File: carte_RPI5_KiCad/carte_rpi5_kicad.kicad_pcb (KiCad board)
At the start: 2 copper layers, 25 parts, among them J0 Vin batterie, J1 Conn_01x03, J2 Conn_01x03, J3 Conn_01x03, J4 Conn_01x03, J5 Conn_01x03, J6 Conn_01x03, J7 Conn_01x03, J8 Conn_01x03, SW1 SW_SPDT

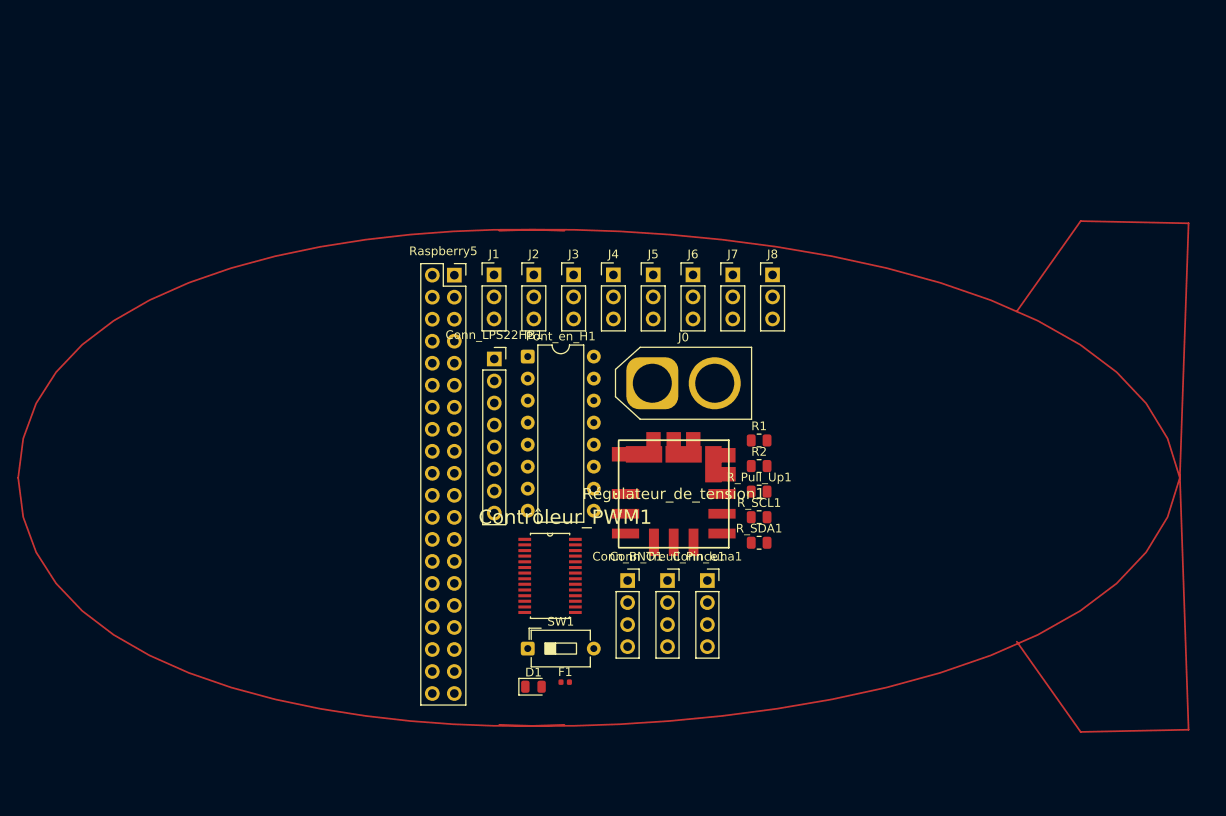
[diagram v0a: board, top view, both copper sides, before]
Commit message: mise à jour PCB
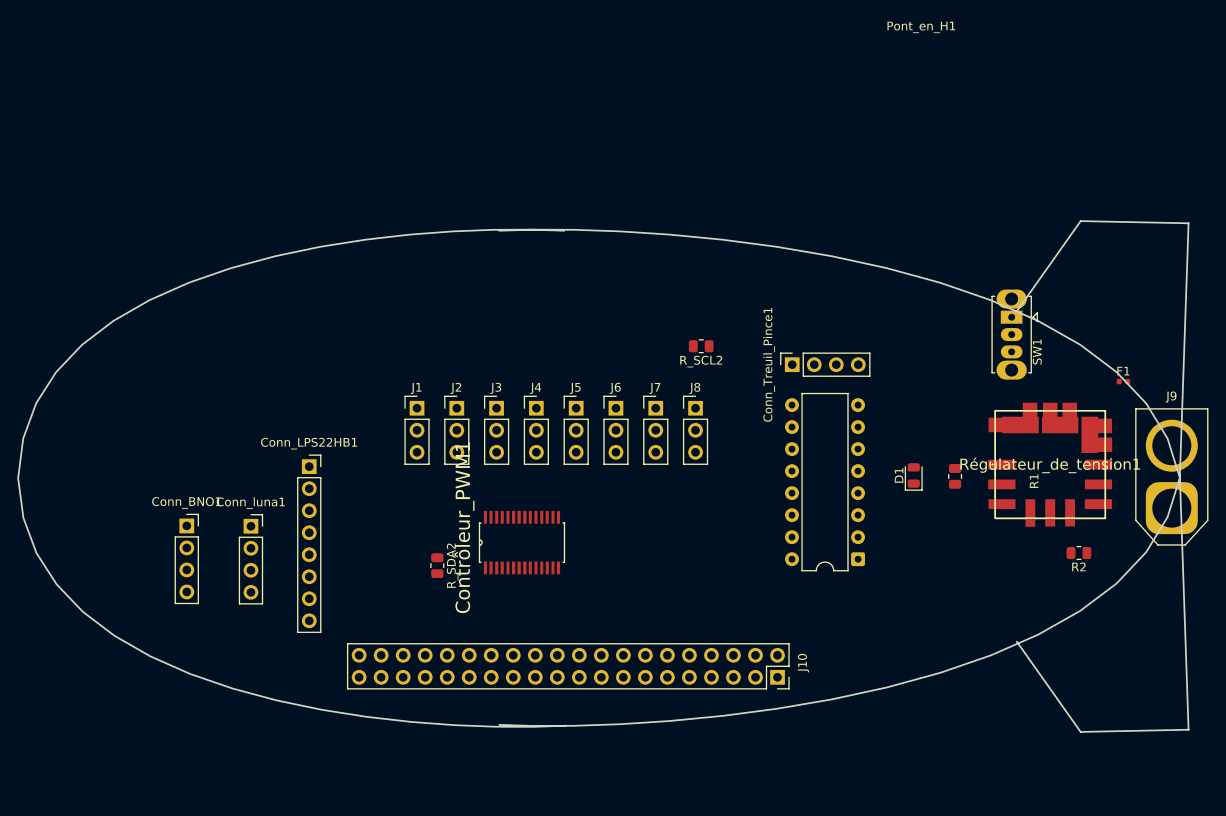
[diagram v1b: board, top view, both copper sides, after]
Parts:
- removed J0: Vin batterie, Connector_AMASS:AMASS_XT60-F_1x02_P7.20mm_Vertical
- removed R_Pull_Up1: 1 k, Resistor_SMD:R_0805_2012Metric
- removed R_SCL1, R_SDA1: 4,7k, Resistor_SMD:R_0805_2012Metric
- removed Raspberry5: CM5108032, Connector_PinSocket_2.54mm:PinSocket_2x20_P2.54mm_Vertical
- added J10: RPI5_40pins, Connector_PinSocket_2.54mm:PinSocket_2x20_P2.54mm_Vertical, F.Cu at (143.6, 109.0)
- added J9: XT60-M, Connector_AMASS:AMASS_XT60-F_1x02_P7.20mm_Vertical, F.Cu at (189.1, 89.5)
- added R_SCL2: 4,7k, Resistor_SMD:R_0805_2012Metric, F.Cu at (134.8, 70.8)
- added R_SDA2: 4,7k, Resistor_SMD:R_0805_2012Metric, F.Cu at (104.3, 96.1)
- SW1: footprint Button_Switch_THT:SW_DIP_SPSTx01_Slide_6.7x4.1mm_W7.62mm_P2.54mm_LowProfile -> Button_Switch_THT:SW_Slide_SPDT_Straight_CK_OS102011MS2Q
- moved F1 73.1 mm to (183.5, 74.9)
- moved SW1 67.7 mm to (170.6, 67.5), turned to -90 degrees
- moved Conn_luna1 53.0 mm to (82.8, 91.6)
- moved Conn_BNO1 51.2 mm to (75.5, 91.5)
- moved D1 50.2 mm to (159.3, 85.7), turned to 90 degrees
- moved Pont_en_H1 44.7 mm to (152.9, 95.4), turned to 180 degrees
- moved Régulateur_de_tension1 43.6 mm to (175.1, 84.5)
- moved R2 38.2 mm to (178.4, 94.7), turned to 180 degrees
- moved Conn_Treuil_Pince1 28.8 mm to (145.3, 73.0), turned to 90 degrees
- moved Conn_LPS22HB1 24.7 mm to (89.6, 84.7)
- moved R1 23.0 mm to (164.1, 85.8), turned to -90 degrees
- moved J5 17.8 mm to (120.4, 78.0)
- moved J6 17.8 mm to (125.0, 78.0)
- moved J1 17.8 mm to (102.0, 78.0)
- moved J2 17.8 mm to (106.6, 78.0)
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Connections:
- SW1 pad 1: Net-(Régulateur_de_tension1-ON/OFF_CONTROL) -> Net-(Régulateur_de_tension1-VIN)
- SW1 pad 2: GND -> Net-(Régulateur_de_tension1-ON/OFF_CONTROL)
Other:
- board outline added: 135 x 58.9 mm

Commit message: Mise à jour du PCB
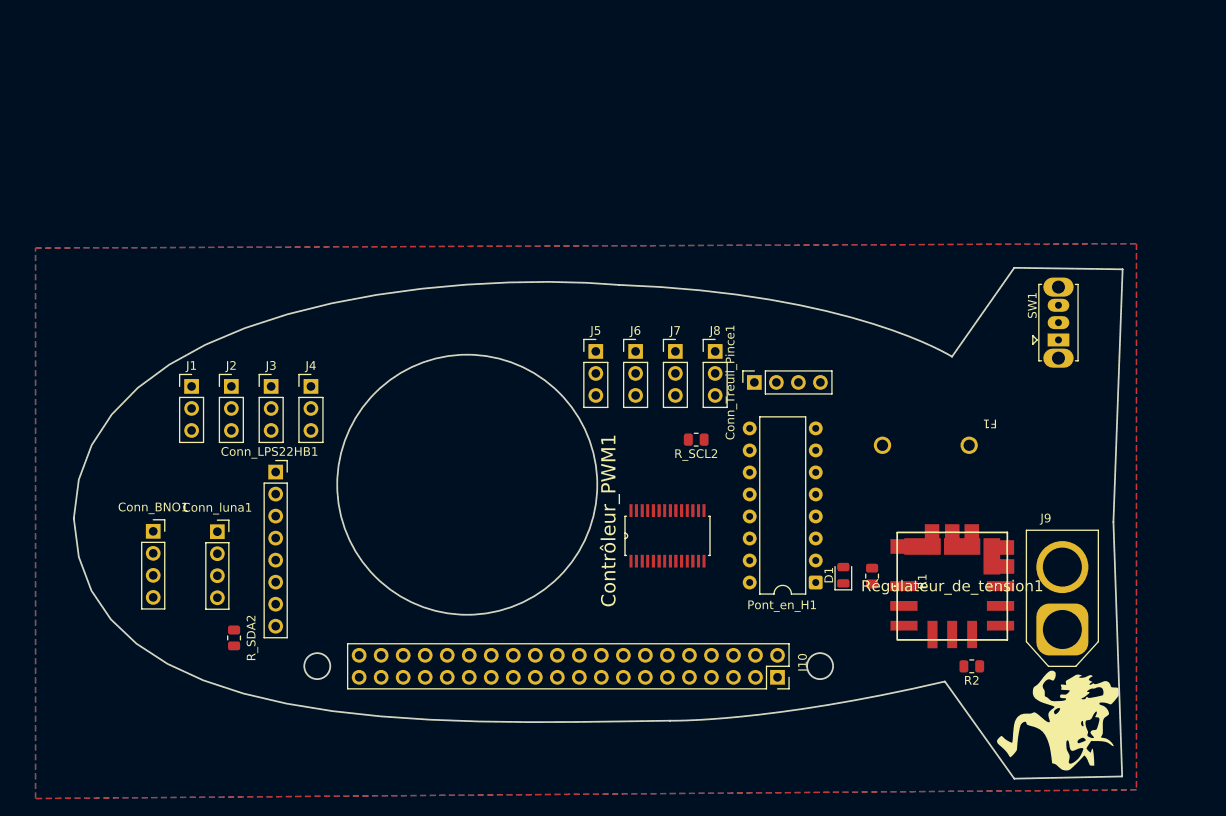
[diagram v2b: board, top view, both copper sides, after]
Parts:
- added ?: , clipboard:6f5e2fe0-dd56-4c47-aeb5-3915356e93c1, F.Cu at (178.7, 114.0)
- F1: footprint Fuse:Fuse_0402_1005Metric -> librairie_empreintes:PTF-50
- moved J4 26.1 mm to (89.8, 75.5)
- moved J1 26.1 mm to (76.0, 75.5)
- moved J2 26.1 mm to (80.6, 75.5)
- moved J3 26.1 mm to (85.2, 75.5)
- moved R_SDA2 24.9 mm to (80.9, 104.5)
- moved J9 18.9 mm to (176.4, 103.5)
- moved Régulateur_de_tension1 18.0 mm to (163.8, 98.5)
- moved R2 18.0 mm to (166.0, 107.8)
- moved Contrôleur_PWM1 16.8 mm to (130.9, 92.7)
- moved F1 16.0 mm to (168.1, 79.2), turned to 180 degrees
- moved R1 15.0 mm to (154.5, 97.3)
- moved D1 14.1 mm to (151.2, 97.2)
- moved R_SCL2 10.8 mm to (134.2, 81.6)
- moved J7 6.94 mm to (131.8, 71.4)
- moved J8 6.94 mm to (136.4, 71.4)
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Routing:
- added copper zone on B.Cu, net GND
- added copper zone on F.Cu, net GND
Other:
- board size 135 x 58.9 mm -> 121 x 58.9 mm
